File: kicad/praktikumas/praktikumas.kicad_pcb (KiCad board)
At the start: 2 copper layers, 39.1 x 37.1 mm, 19 parts, among them J1 sp, J2 Conn_01x01_Socket, J3 sp, Q1 2n3904, Q2 2n3904, U2 LM386

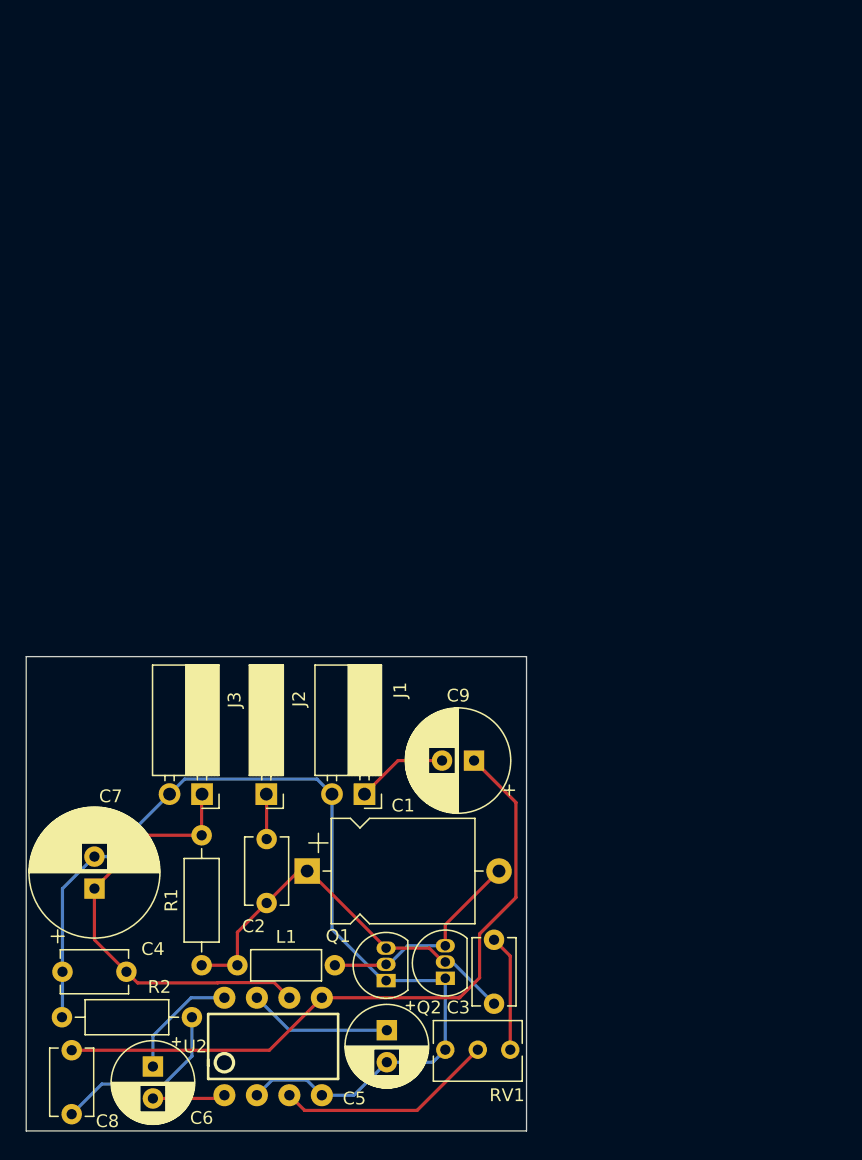
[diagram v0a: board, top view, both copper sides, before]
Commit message: 9
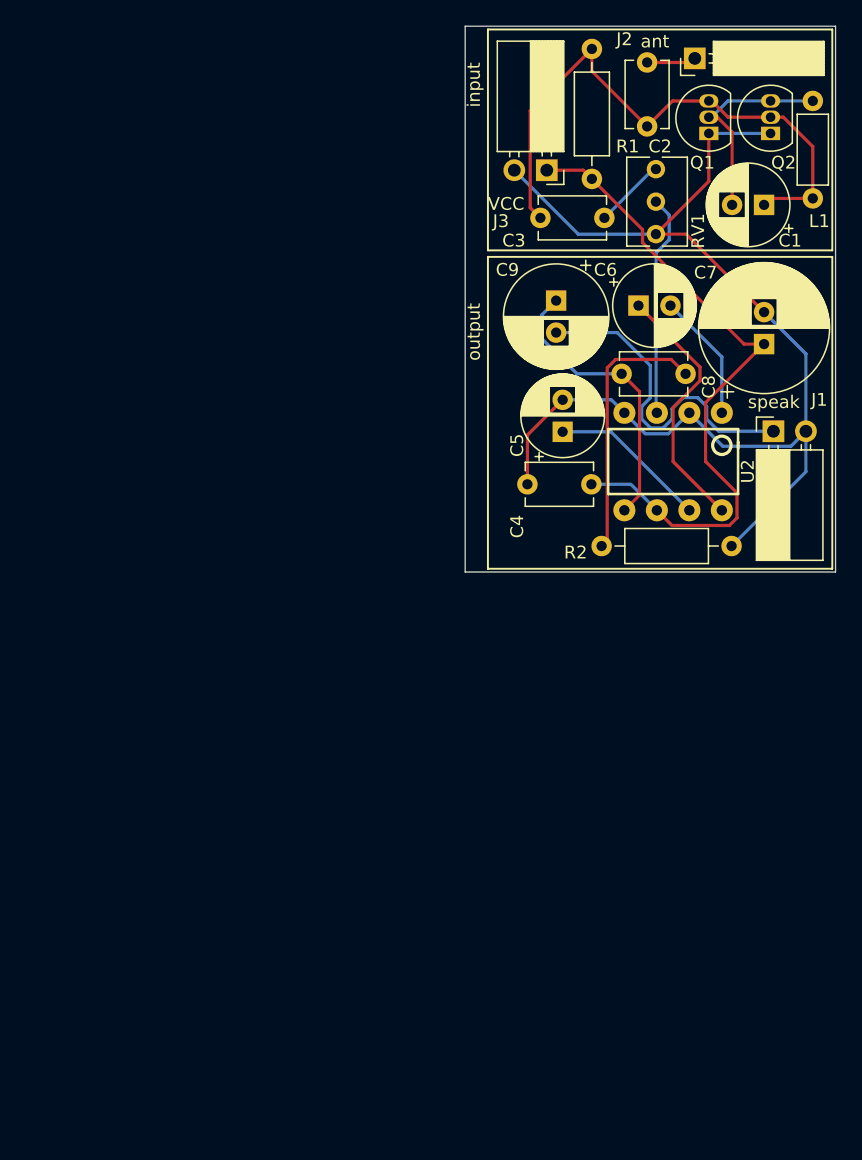
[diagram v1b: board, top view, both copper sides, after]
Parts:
- C1: footprint Capacitor_THT:CP_Axial_L11.0mm_D8.0mm_P15.00mm_Horizontal -> Capacitor_THT:CP_Radial_D6.3mm_P2.50mm
- moved R1 77.9 mm to (181.6, 36.1), turned to -90 degrees
- moved C8 75.2 mm to (188.9, 61.5), turned to 180 degrees
- moved L1 75.0 mm to (198.9, 47.8), turned to 90 degrees
- moved Q1 70.9 mm to (190.8, 42.7)
- moved Q2 70.8 mm to (195.6, 42.7)
- moved C6 70.6 mm to (185.3, 56.1), turned to 0 degrees
- moved RV1 69.8 mm to (186.6, 45.5), turned to 90 degrees
- moved C2 67.6 mm to (185.9, 42.1)
- moved C7 67.5 mm to (195.1, 59.1)
- moved J2 66.6 mm to (189.7, 36.8), turned to 180 degrees
- moved R2 64.0 mm to (192.5, 74.9), turned to 180 degrees
- moved C1 63.2 mm to (195.1, 48.3), turned to 180 degrees
- moved C3 61.5 mm to (177.6, 49.3), turned to 0 degrees
- moved J3 55.7 mm to (178.1, 45.5)
- moved U2 55.4 mm to (188.0, 68.3), turned to 180 degrees
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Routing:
- net Net-(C8-Pad2): track 53.8 -> 23.8 mm
- net Net-(J1-Pin_1): track 7.15 -> 26.6 mm
- net +5V: track 34.5 -> 52.7 mm
- net Net-(Q1-E): track 31.7 -> 46.7 mm
- net GND: track 79.4 -> 90.7 mm
- net Net-(C6-Pad1): track 9.22 -> 20.4 mm
- net Net-(C8-Pad1): track 14.3 -> 21.0 mm
- net Net-(C6-Pad2): track 5.69 -> 10.0 mm
- net Net-(C3-Pad2): track 9.12 -> 5.61 mm
- net Net-(C5-Pad1): track 11.2 -> 12.4 mm
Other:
- board size 39.1 x 37.1 mm -> 29 x 42.7 mm
- board text added: "VCC"
- board text added: "ant"
- board text added: "input"
- board text added: "output"
- board text added: "speak"
